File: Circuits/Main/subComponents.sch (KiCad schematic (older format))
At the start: 76 parts

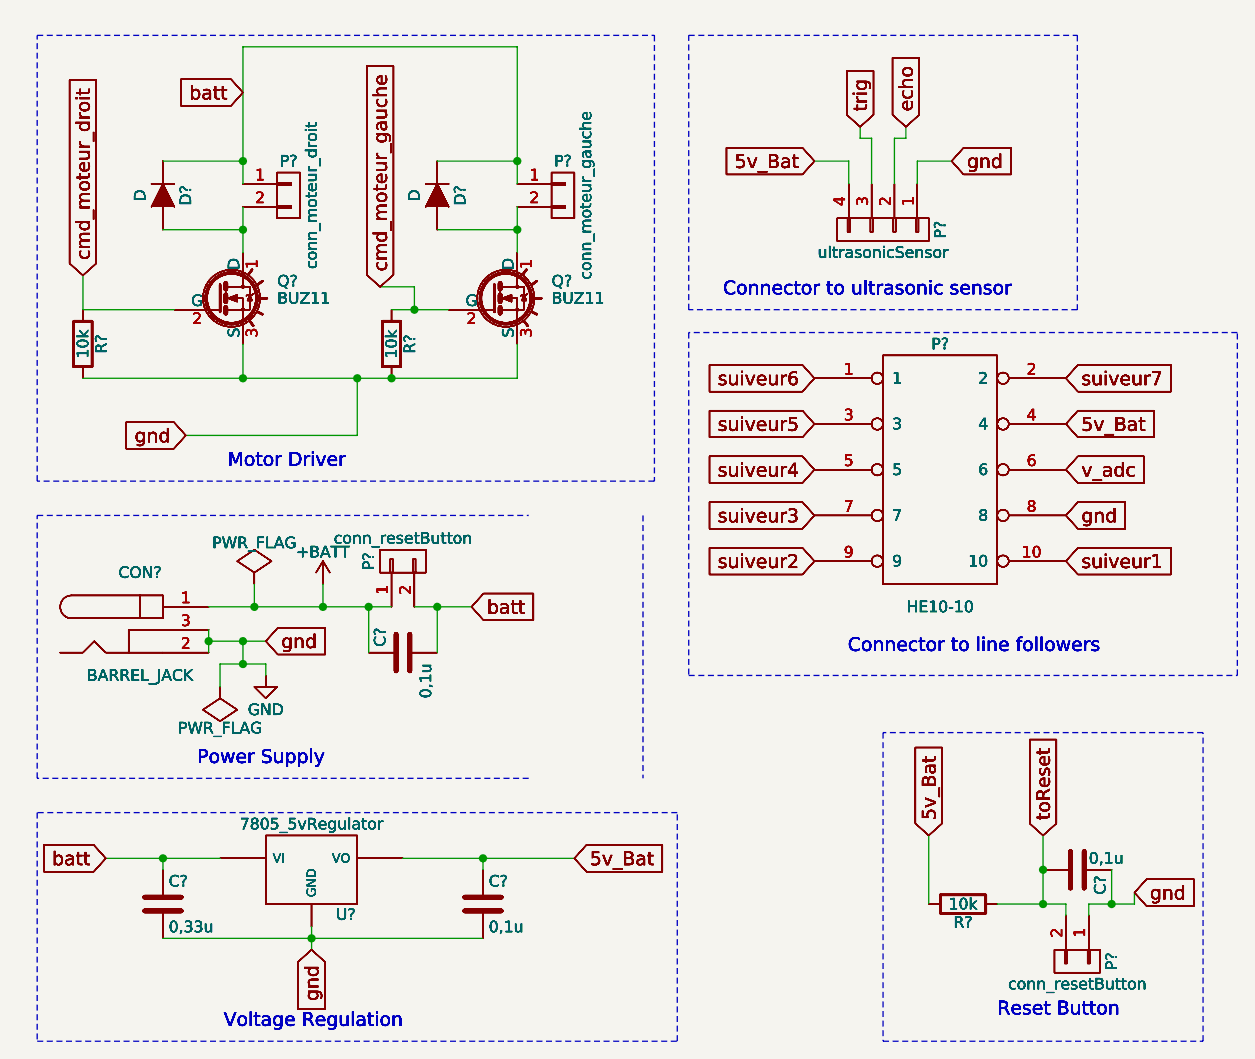
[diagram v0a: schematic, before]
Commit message: Ameliorations cartes + rapport
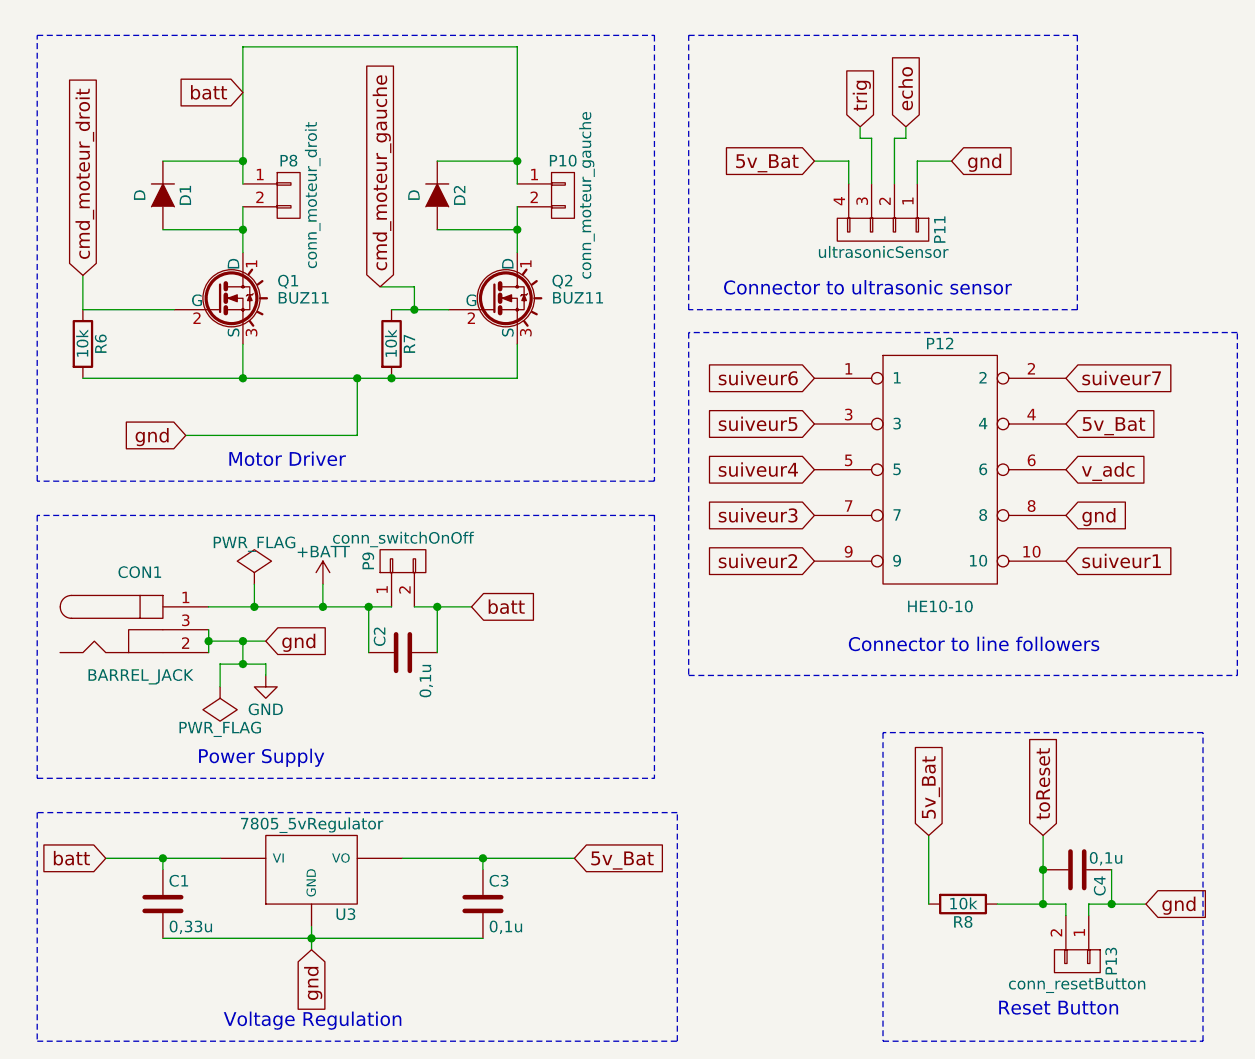
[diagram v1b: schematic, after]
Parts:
- removed C? (x3): 0,33u, Capacitors_ThroughHole:C_Disc_D3_P2.5, symbol C
- removed C? (x9): 0,1u, Capacitors_ThroughHole:C_Disc_D3_P2.5, symbol C
- removed CON? (x3): BARREL_JACK, Connect:BARREL_JACK, symbol BARREL_JACK
- removed D? (x6): D, Diodes_ThroughHole:Diode_DO-35_SOD27_Horizontal_RM10, symbol D
- removed P? (x3): conn_moteur_droit, Pin_Headers:Pin_Header_Straight_1x02, symbol CONN_01X02
- removed P? (x3): conn_moteur_gauche, Pin_Headers:Pin_Header_Straight_1x02, symbol CONN_01X02
- removed P? (x3): HE10-10, Connect:he10-10d, symbol HE10-10
- removed P? (x3): ultrasonicSensor, Pin_Headers:Pin_Header_Straight_1x04, symbol CONN_01X04
- removed P? (x6): conn_resetButton, Pin_Headers:Pin_Header_Straight_1x02, symbol CONN_01X02
- removed Q? (x6): BUZ11, Power_Integrations:TO-220, symbol BUZ11
- removed R? (x9): 10k, Resistors_ThroughHole:Resistor_Horizontal_RM10mm, symbol R
- removed U? (x3): 7805_5vRegulator, MES_EMPREINTES:voltageRegulator5v, symbol 7805_5vRegulator
- P9: renamed from P?; value conn_resetButton -> conn_switchOnOff
- gave numbers to parts that had none: 18
